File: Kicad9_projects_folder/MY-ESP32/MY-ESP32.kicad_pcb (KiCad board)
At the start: 4 copper layers, 90.5 x 104.2 mm, 90 parts, among them J1 SM04B-SRSS-TB, J2 SM04B-SRSS-TB, Q1 2N3904S-RTK/PS, Q10 N-MOSFET-ENH-2N7002, Q2 2N3904S-RTK/PS, Q3 N-MOSFET-ENH-2N7002, Q4 P-MOSFET-ENH-BSS84LT1G, Q5 PMOSFET-DMP1045U-7, Q7 N-MOSFET-ENH-2N7002, Q8 P-MOSFET-ENH-BSS84LT1G, Q9 P-MOSFET-ENH-BSS84LT1G, SW3 SPDT, U1 USBLC6-2SC6, U3 CP2102N-Axx-xQFN28, U4 DFR0819, U5 TPS63001DRCR, U7 USB4110GFA

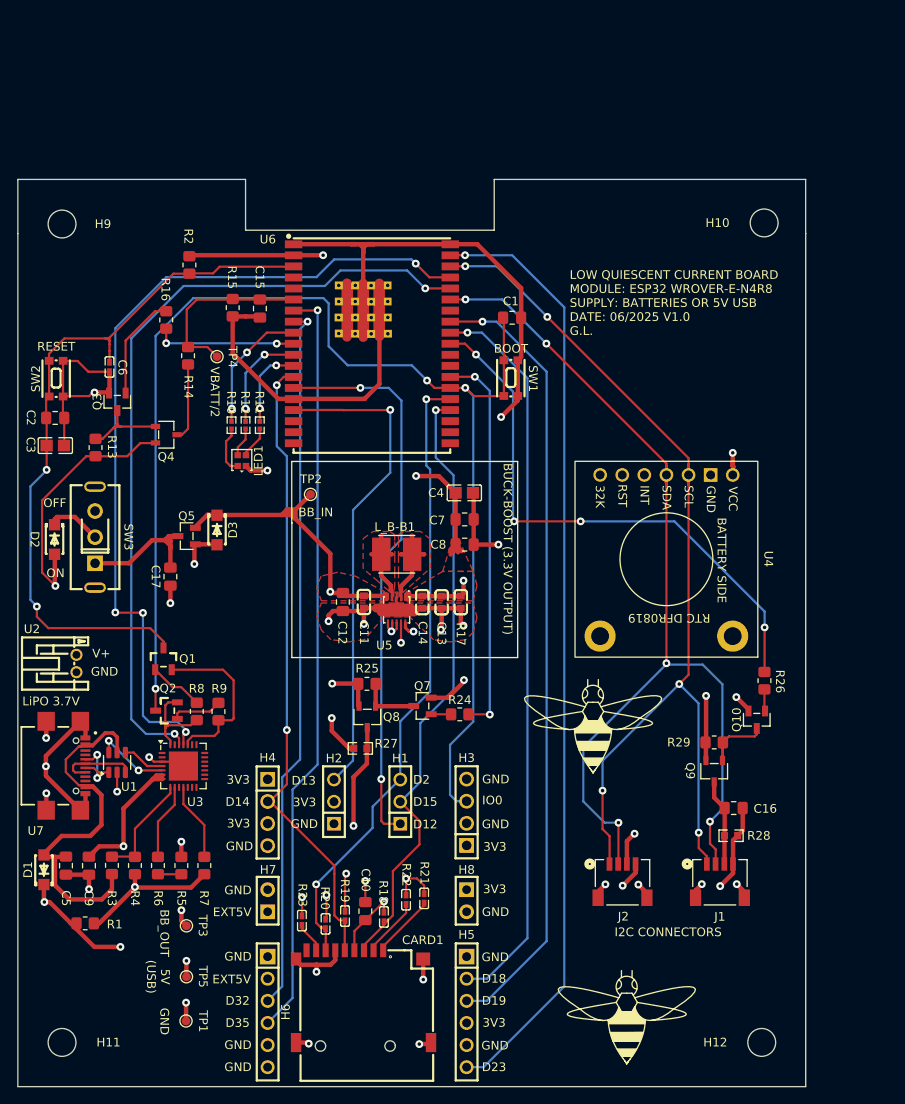
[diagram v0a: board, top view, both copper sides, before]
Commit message: 5th commit
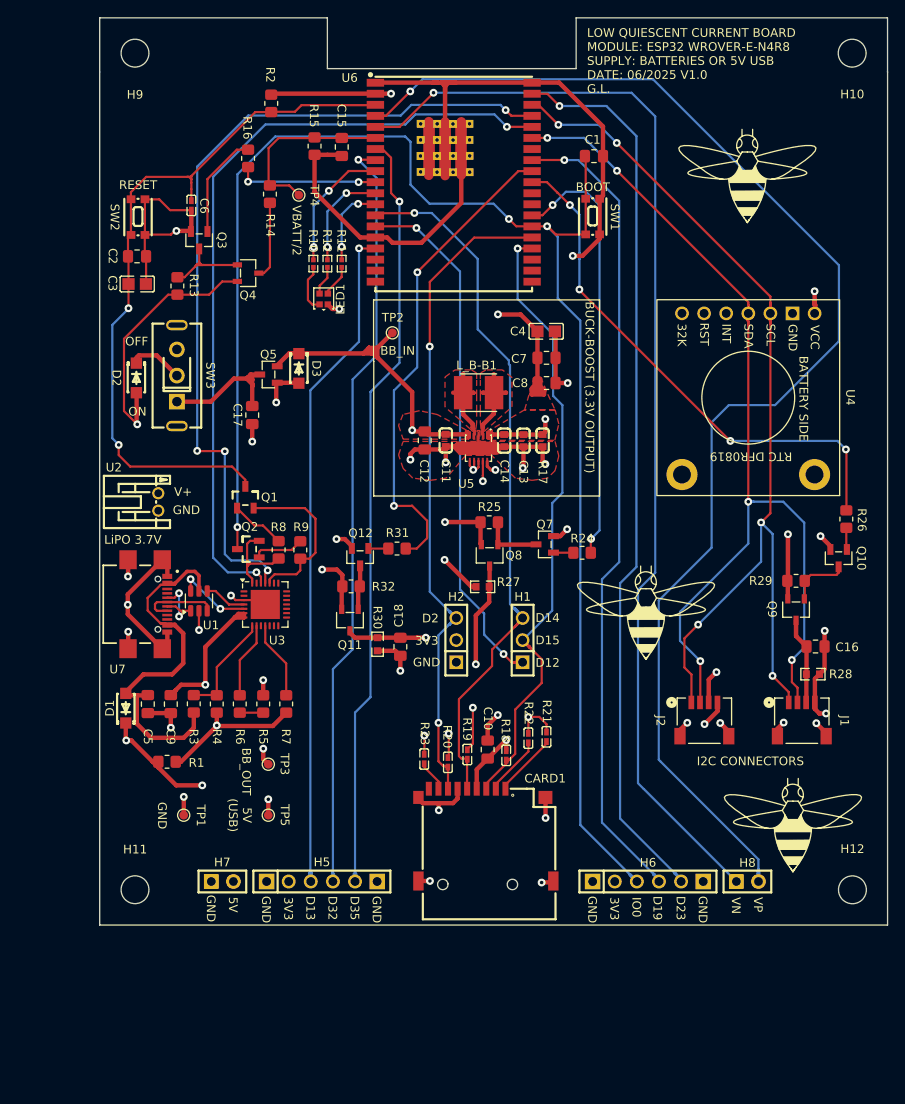
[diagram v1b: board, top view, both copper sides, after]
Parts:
- removed H3, H4: Header-Female-2.54_1x4, My_Personal_Footprints_Library:Header-Female-2.54_1x4
- added C18: 104, Capacitor_SMD:C_0805_2012Metric_Pad1.18x1.45mm_HandSolder, F.Cu at (129.5, 106.9)
- added Q11: P-MOSFET-ENH-BSS84LT1G, My_Personal_Footprints_Library:BSS84LT1G, F.Cu at (123.8, 103.8)
- added Q12: N-MOSFET-ENH-2N7002, My_Personal_Footprints_Library:2N7002, F.Cu at (124.9, 96.6)
- added R30: 4.7kΩ ±1% 100mW, My_Personal_Footprints_Library:0603WAF4701T5E, F.Cu at (126.9, 106.6)
- added R31: 100, Resistor_SMD:R_0805_2012Metric_Pad1.20x1.40mm_HandSolder, F.Cu at (129.2, 95.6)
- added R32: 10K, Resistor_SMD:R_0805_2012Metric_Pad1.20x1.40mm_HandSolder, F.Cu at (123.9, 99.9)
- added REF**: BEE_LOGO, My_Personal_Footprints_Library:BEE_LOGO, F.Cu at (169.4, 52.5)
- moved H6 46.2 mm to (158.0, 133.8), turned to 0 degrees
- moved H8 32.3 mm to (169.4, 133.8), turned to 0 degrees
- moved TP1 23.6 mm to (104.7, 126.2)
- moved C10 23.3 mm to (139.6, 118.7)
- moved CARD1 23.3 mm to (139.4, 128.5)
- moved H1 23.3 mm to (143.6, 106.1)
- moved H2 23.3 mm to (136.0, 106.1)
- moved Q8 23.3 mm to (139.8, 96.4)
- moved R18 23.3 mm to (141.7, 119.3)
- moved R21 23.3 mm to (146.3, 117.2)
- moved R23 23.3 mm to (132.3, 119.8)
- moved Q7 23.3 mm to (146.1, 95.1)
- moved R19 23.3 mm to (137.2, 119.2)
- moved R22 23.3 mm to (144.3, 117.4)
- moved R24 23.3 mm to (150.4, 96.1)
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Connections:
- H1 pad 3: D2 -> D14
- H2 pad 2: +3V3 -> 3V3_ON_OFF
- H2 pad 3: D13 -> D2
- H5 pad 2: D18 -> 3V3_ON_OFF
- H5 pad 3: D19 -> D13
- H5 pad 4: +3V3 -> D32
- H5 pad 5: GND -> D35
- H5 pad 6: D23 -> GND
- H6 pad 2: EXT_5V -> +3V3
- H6 pad 3: D32 -> IO0
- H6 pad 4: D35 -> D19
- H6 pad 5: GND -> D23
- H7 pad 1: EXT_5V -> GND
- H7 pad 2: GND -> EXT_5V
- H8 pad 1: +3V3 -> SENSOR_VN
- H8 pad 2: GND -> SENSOR_VP
- U6 pad 4: unconnected-(U6-SENSOR_VP-Pad4) -> SENSOR_VP
- U6 pad 5: unconnected-(U6-SENSOR_VN-Pad5) -> SENSOR_VN
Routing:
- net SENSOR_VP: track 0.00 -> 151.9 mm, vias 0 -> 1
- net SENSOR_VN: track 0.00 -> 127.3 mm, vias 0 -> 1
- net 3V3_ON_OFF: track 0.00 -> 47.9 mm, vias 0 -> 1
- net IO0: track 151.1 -> 181.2 mm
- net D18: track 83.8 -> 55.5 mm, vias 1 -> 2
- net +3V3: track 384.1 -> 359.6 mm, vias 12 -> 13
- net D13: track 55.5 -> 77.3 mm
- net GND: track 267.7 -> 282.4 mm, vias 31 -> 34
- net D14: track 71.9 -> 82.3 mm, vias 2 -> 1
- net EXT_5V: track 104.2 -> 93.9 mm
- net D32: track 80.8 -> 88.8 mm
- net Net-(Q11-G): track 0.00 -> 5.09 mm
- net D4: track 44.8 -> 49.8 mm
- net D2: track 71.5 -> 76.1 mm
- net D23: track 107.9 -> 103.4 mm
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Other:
- board text added: "5V"
- board text added: "VN"
- board text added: "VP"
- board text removed: "D18"
- board text removed: "EXT5V"

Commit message: 5th commit
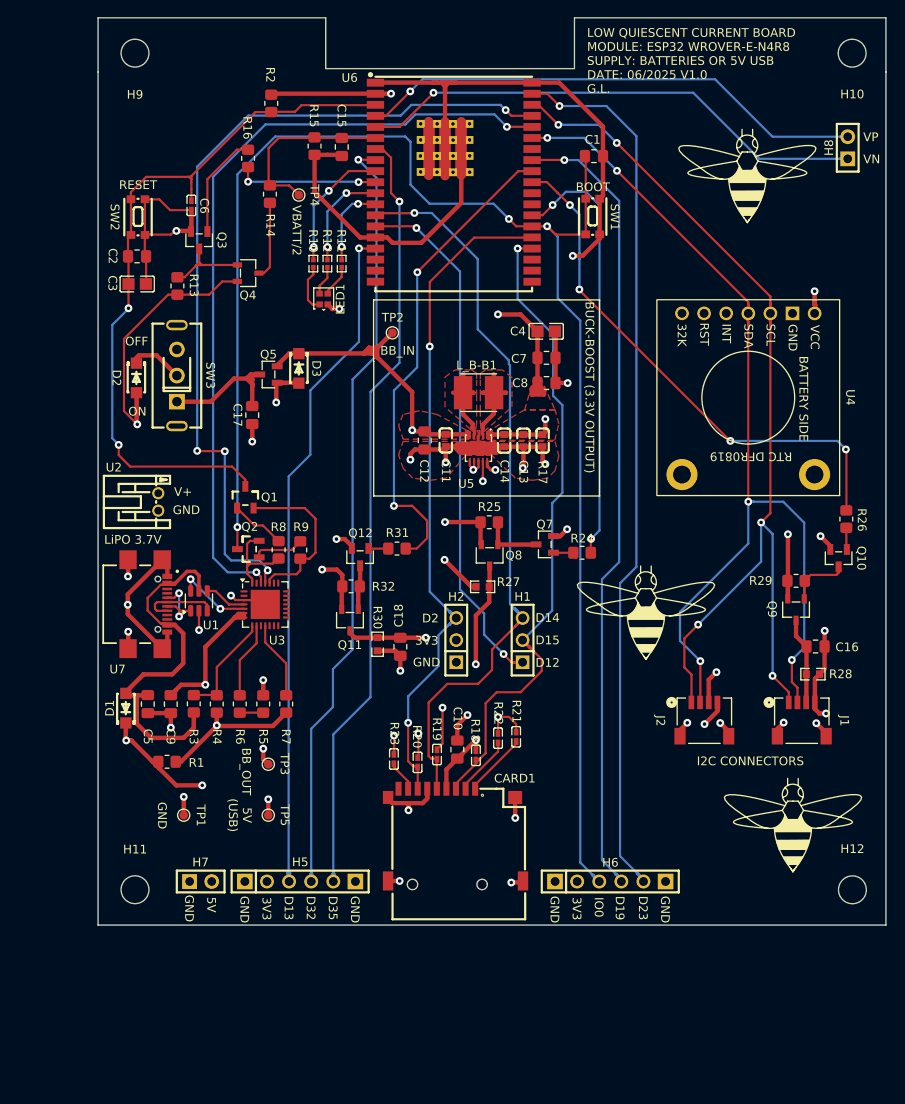
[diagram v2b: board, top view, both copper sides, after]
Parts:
- moved H8 85.1 mm to (180.9, 49.5), turned to 90 degrees
- moved H6 4.32 mm to (153.7, 133.8)
- moved CARD1 3.48 mm to (135.9, 128.5)
- moved R21 3.48 mm to (142.9, 117.2)
- moved R23 3.48 mm to (128.8, 119.8)
- moved C10 3.48 mm to (136.1, 118.7)
- moved R18 3.48 mm to (138.2, 119.3)
- moved R19 3.48 mm to (133.8, 119.2)
- moved R20 3.48 mm to (131.5, 120.1)
- moved R22 3.48 mm to (140.8, 117.4)
- moved H5 2.50 mm to (118.0, 133.8)
- moved H7 2.50 mm to (106.6, 133.8)
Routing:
- net SENSOR_VP: track 151.9 -> 57.9 mm
- net SENSOR_VN: track 127.3 -> 58.3 mm
- net D14: track 82.3 -> 85.8 mm
- net D15: track 71.6 -> 74.6 mm
- net +3V3: track 359.6 -> 361.4 mm
- net D23: track 103.4 -> 101.6 mm
- net IO0: track 181.2 -> 179.4 mm
- net D19: track 93.4 -> 91.6 mm
- net D2: track 76.1 -> 77.6 mm
- net /micro_SD-CARD_enable/3V3_Input_to_micro_SD-CARD: track 68.6 -> 67.1 mm
- net EXT_5V: track 93.9 -> 95.0 mm
- net D32: track 88.8 -> 89.9 mm
- net D35: track 88.5 -> 89.5 mm
- net D13: track 77.3 -> 78.4 mm
- net 3V3_ON_OFF: track 47.9 -> 49.0 mm
